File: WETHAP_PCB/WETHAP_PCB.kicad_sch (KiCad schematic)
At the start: 9 parts, among them J1 Conn_01x20_Socket, J2 Conn_01x20_Socket

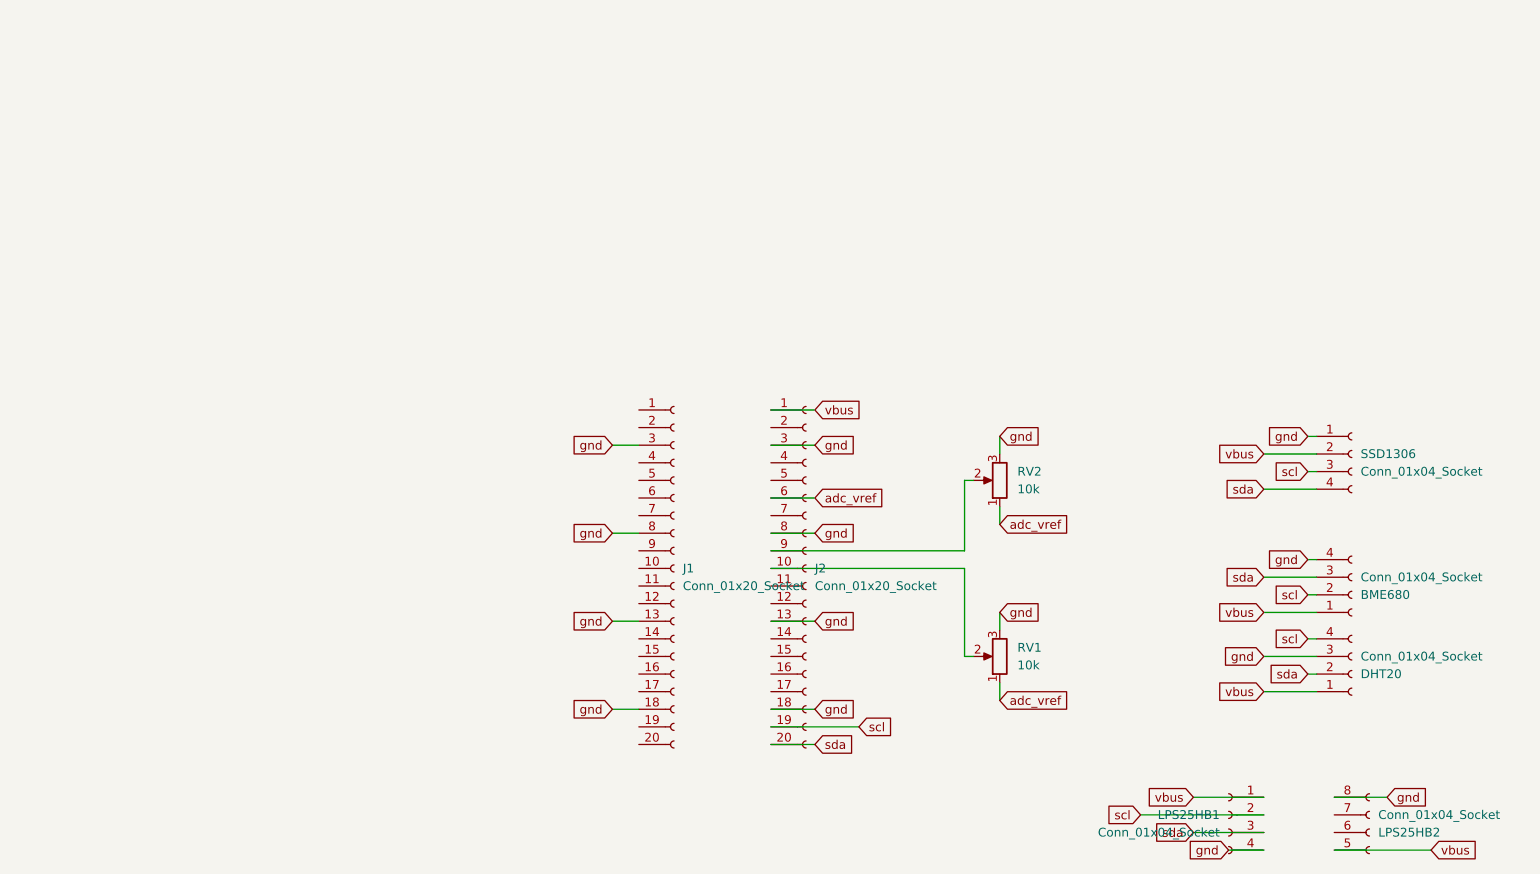
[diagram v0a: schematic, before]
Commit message: websocket
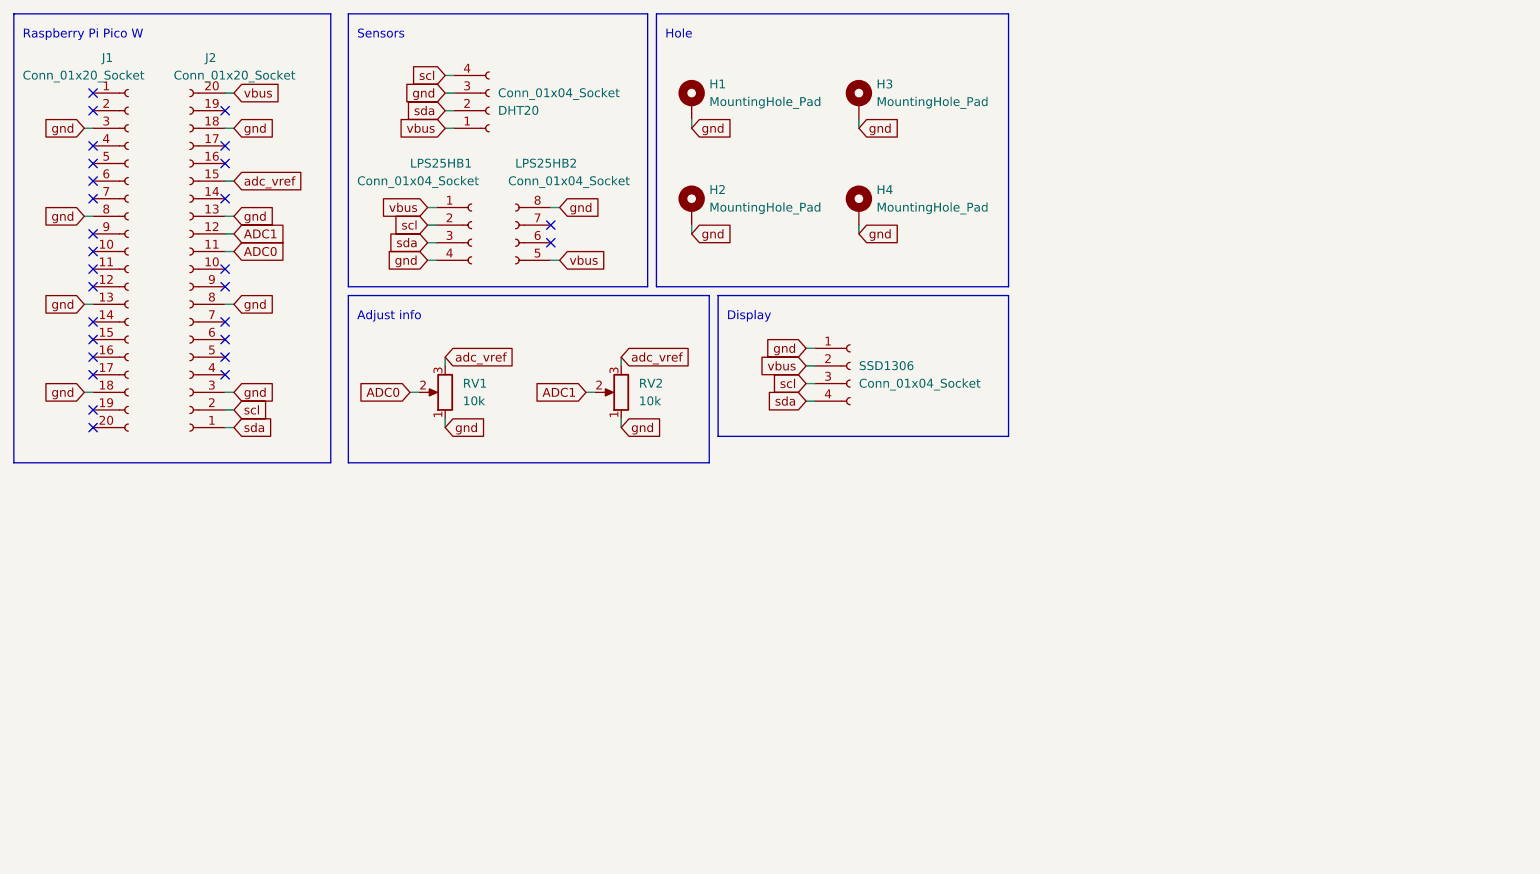
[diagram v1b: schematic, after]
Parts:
- removed BME680: Conn_01x04_Socket, Connector_PinHeader_2.54mm:PinHeader_1x04_P2.54mm_Vertical, symbol Connector:Conn_01x04_Socket
- added H1, H2, H3, H4: MountingHole_Pad, MountingHole:MountingHole_3.2mm_M3_DIN965_Pad, symbol Mechanical:MountingHole_Pad
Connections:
- net adc_vref: now also J2.15 (Pin_15), RV1.3, RV2.3; no longer J2.6 (Pin_6), RV1.1, RV2.1
- net gnd: now also RV1.1, RV2.1, H1.1, H2.1, H3.1, H4.1; no longer RV1.3, RV2.3
- net scl: now also J2.2 (Pin_2); no longer J2.19 (Pin_19)
- net sda: now also J2.1 (Pin_1); no longer J2.20 (Pin_20)
- net vbus: now also J2.20 (Pin_20); no longer J2.1 (Pin_1)
- net at J2.10 (Pin_10): no longer RV1.2
- net ADC0: now reaches J2.11 (Pin_11)
- net ADC0: now also RV1.2
- net ADC1: now reaches J2.12 (Pin_12)
- net ADC1: now also RV2.2
- net at J2.9 (Pin_9): no longer RV2.2
- no-connect marks 0 -> 28
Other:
- note added: "Adjust info"
- note added: "Display"
- note added: "Hole"
- note added: "Raspberry Pi Pico W"
- note added: "Sensors"
- moved on the sheet: DHT20, J1, J2, LPS25HB1, LPS25HB2, RV1, RV2, SSD1306
